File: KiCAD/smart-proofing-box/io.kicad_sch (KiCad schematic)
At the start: 6 parts, among them SW3 UP, SW4 DOWN, SW5 SW_LEFT, SW6 SW_RIGHT, SW7 SW_SELECT, U4 TCA9535PWR

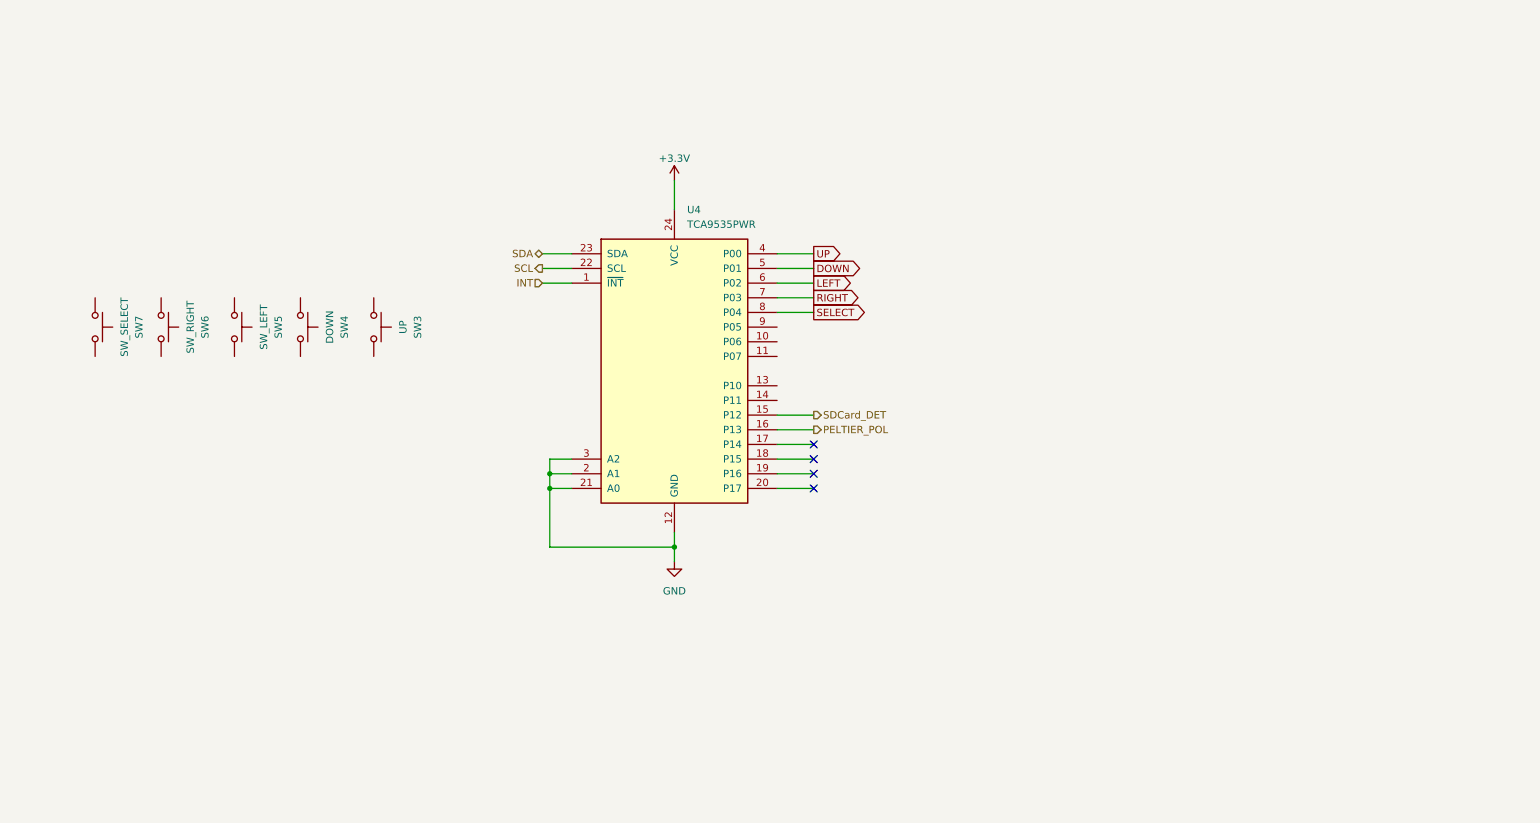
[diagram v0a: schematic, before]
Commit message: continued work on schematic
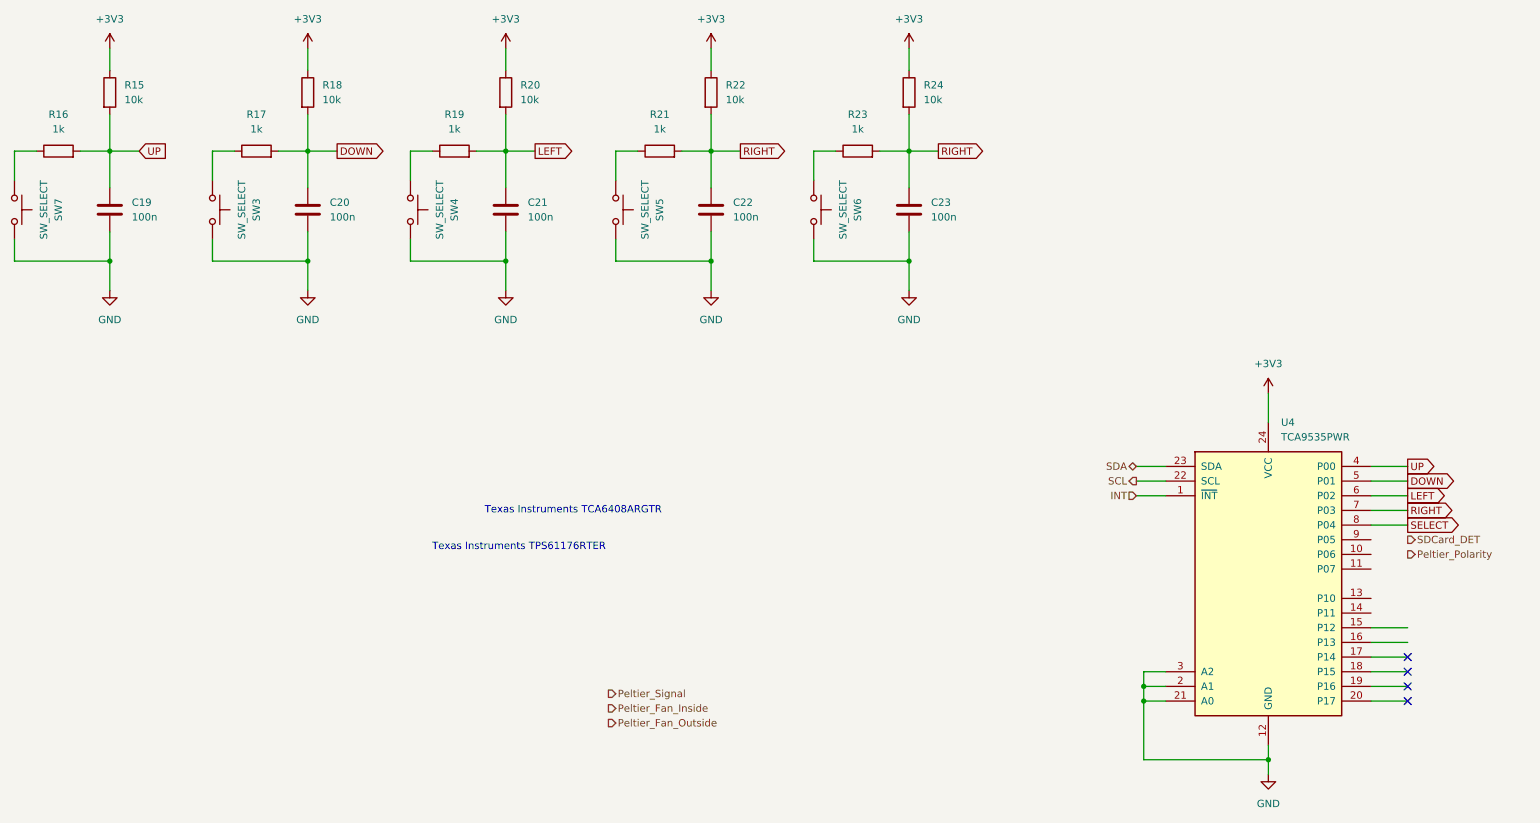
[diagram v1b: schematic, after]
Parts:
- added C19, C20, C21, C22, C23: 100n, Capacitor_SMD:C_0402_1005Metric_Pad0.74x0.62mm_HandSolder, symbol Device:C
- added R15, R18, R20, R22, R24: 10k, Resistor_SMD:R_0402_1005Metric_Pad0.72x0.64mm_HandSolder, symbol Device:R
- added R16, R17, R19, R21, R23: 1k, Resistor_SMD:R_0402_1005Metric_Pad0.72x0.64mm_HandSolder, symbol Device:R
- SW3: value UP -> SW_SELECT
- SW4: value DOWN -> SW_SELECT
- SW5: value SW_LEFT -> SW_SELECT
- SW6: value SW_RIGHT -> SW_SELECT
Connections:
- net DOWN: now also C20.1, R17.2, R18.2
- net GND: now also SW3.2, SW4.2, SW5.2, SW6.2, SW7.2, C19.2, C20.2, C21.2, C22.2, C23.2
- net LEFT: now also C21.1, R19.2, R20.2
- net RIGHT: now also C22.1, C23.1, R21.2, R22.2, R23.2, R24.2
- net SDCard_DET: no longer U4.15 (P12)
- net UP: now also C19.1, R15.2, R16.2
- net at SW3.1: now also R17.1
- net at SW4.1: now also R19.1
- net at SW7.1: now also R16.1
- net at SW5.1: now also R21.1
- net at SW6.1: now also R23.1
- net +3.3V renamed +3V3
- net +3V3: now also R15.1, R18.1, R20.1, R22.1, R24.1
- net PELTIER_POL: no longer names the net of U4.16 (P13)
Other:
- note added: "Texas Instruments TCA6408ARGTR"
- note added: "Texas Instruments TPS61176RTER"
- moved on the sheet: SW7, U4
